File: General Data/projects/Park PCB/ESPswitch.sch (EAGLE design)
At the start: 9 parts, among them T1 2N2222, T2 2N2222

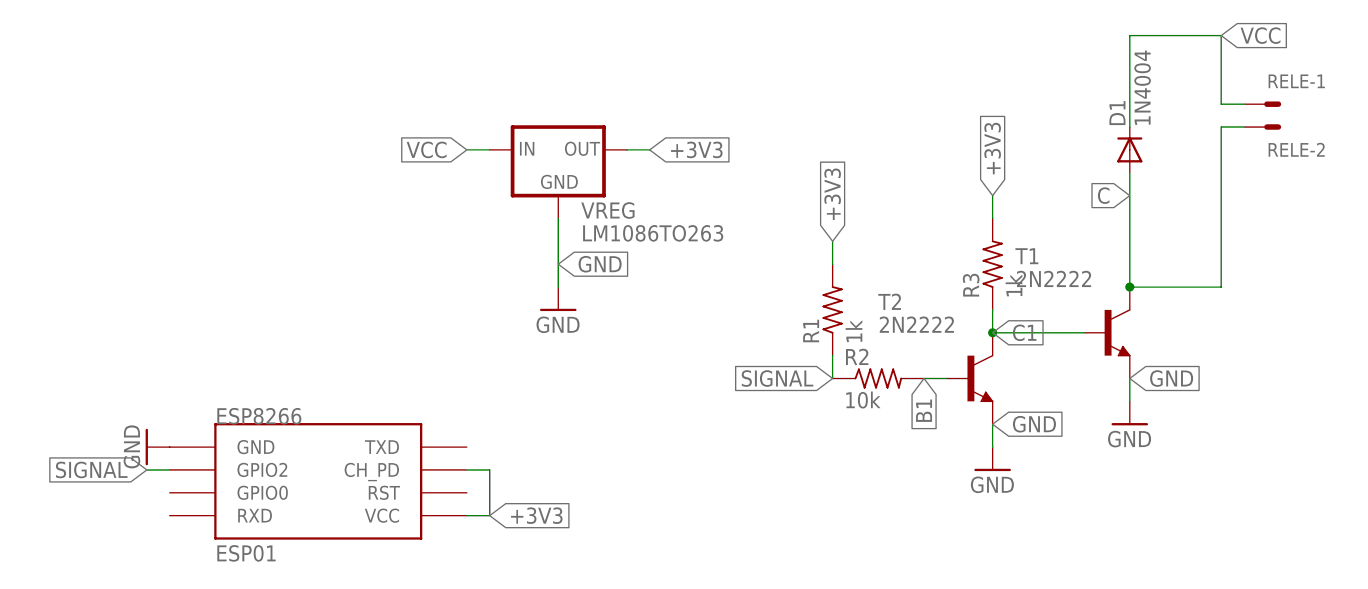
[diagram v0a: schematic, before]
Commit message: Actualización de PCBs
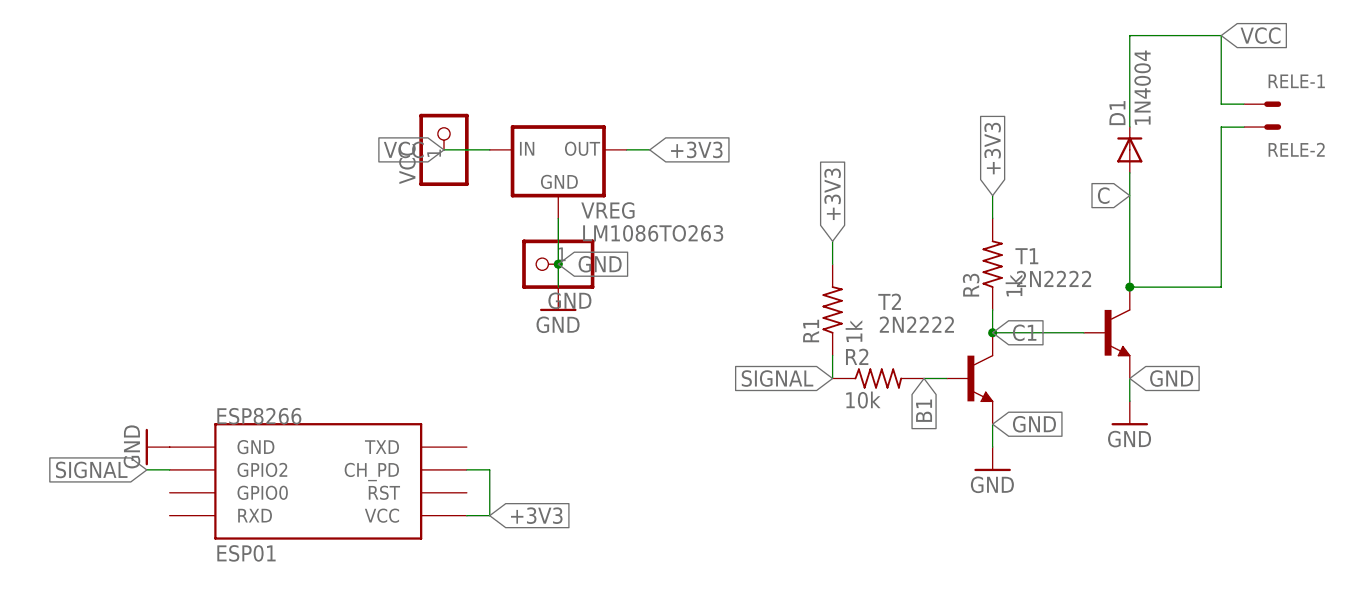
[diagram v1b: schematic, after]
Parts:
- added GND, VCC: (no value), adafruit:PINHD-1X1
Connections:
- net GND: now also GND.1
- net VCC: now also VCC.1
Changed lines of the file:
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@@
 <part name="GND3" library="supply1" library_urn="urn:adsk.eagle:library:371" deviceset="GND" device=""/>
 <part name="GND4" library="supply1" library_urn="urn:adsk.eagle:library:371" deviceset="GND" device=""/>
+<part name="VCC" library="adafruit" library_urn="urn:adsk.eagle:library:420" deviceset="PINHD-1X1" device="" package3d_urn="urn:adsk.eagle:package:6240654/1"/>
+<part name="GND" library="adafruit" library_urn="urn:adsk.eagle:library:420" deviceset="PINHD-1X1" device="" package3d_urn="urn:adsk.eagle:package:6240654/1"/>
 </parts>
 <sheets>
@@
 <attribute name="VALUE" x="0" y="99.06" size="1.778" layer="96"/>
 </instance>
+<instance part="VCC" gate="G$1" x="-10.16" y="121.92" smashed="yes" rot="R90">
+<attribute name="NAME" x="-13.335" y="115.57" size="1.778" layer="95" rot="R90"/>
+<attribute name="VALUE" x="-5.08" y="115.57" size="1.778" layer="96" rot="R90"/>
+</instance>
+<instance part="GND" gate="G$1" x="0" y="106.68" smashed="yes" rot="R180">
+<attribute name="NAME" x="6.35" y="103.505" size="1.778" layer="95" rot="R180"/>
+<attribute name="VALUE" x="6.35" y="111.76" size="1.778" layer="96" rot="R180"/>
+</instance>
 </instances>
 <busses>
@@
 <segment>
 <pinref part="VREG" gate="G$1" pin="GND"/>
-<wire x1="2.54" y1="104.14" x2="2.54" y2="111.76" width="0.1524" layer="91"/>
+<wire x1="2.54" y1="104.14" x2="2.54" y2="106.68" width="0.1524" layer="91"/>
 <label x="2.54" y="106.68" size="1.778" layer="95" xref="yes"/>
 <pinref part="GND4" gate="1" pin="GND"/>
+<pinref part="GND" gate="G$1" pin="1"/>
+<wire x1="2.54" y1="106.68" x2="2.54" y2="111.76" width="0.1524" layer="91"/>
+<junction x="2.54" y="106.68"/>
 </segment>
 <segment>
@@
 <segment>
 <pinref part="VREG" gate="G$1" pin="IN"/>
-<wire x1="-5.08" y1="119.38" x2="-7.62" y2="119.38" width="0.1524" layer="91"/>
-<label x="-7.62" y="119.38" size="1.778" layer="95" rot="R180" xref="yes"/>
+<wire x1="-5.08" y1="119.38" x2="-10.16" y2="119.38" width="0.1524" layer="91"/>
+<label x="-10.16" y="119.38" size="1.778" layer="95" rot="R180" xref="yes"/>
+<pinref part="VCC" gate="G$1" pin="1"/>
 </segment>
 </net>
